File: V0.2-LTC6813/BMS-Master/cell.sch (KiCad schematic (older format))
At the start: 3 parts

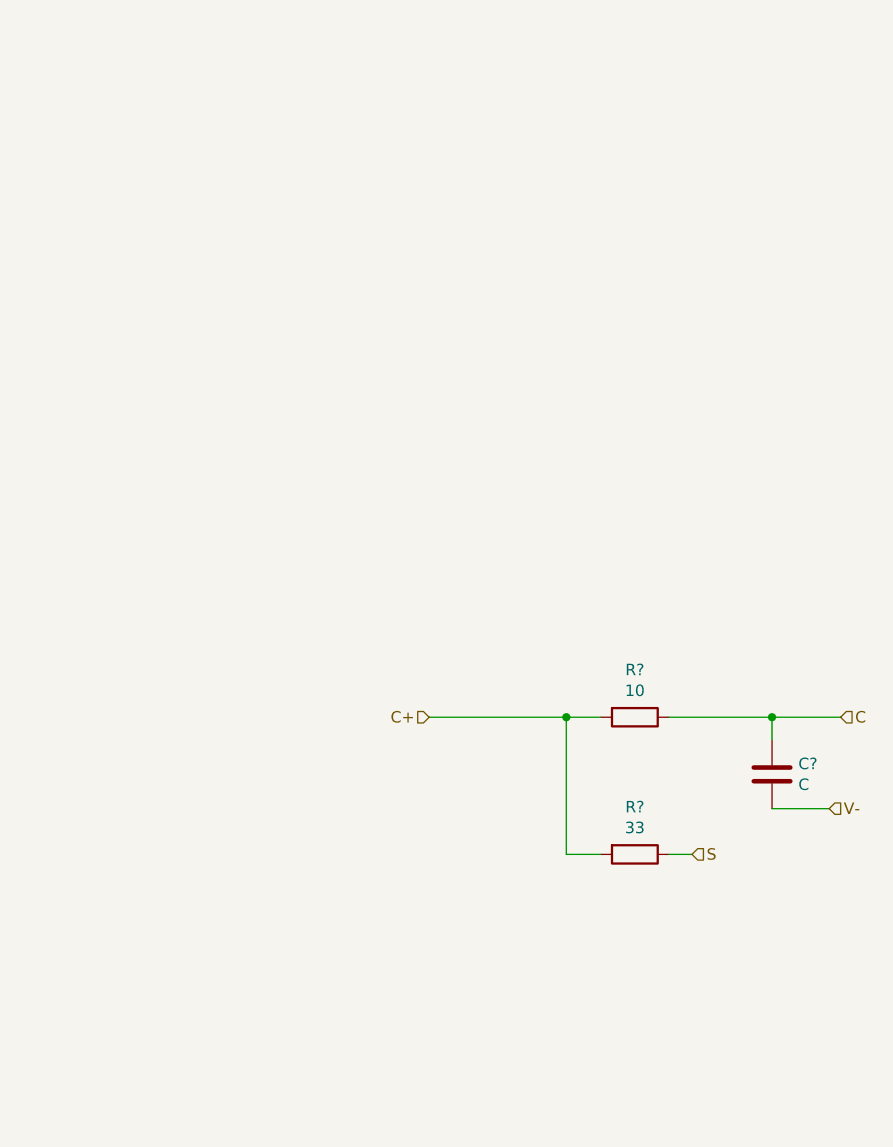
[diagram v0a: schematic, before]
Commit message: schematics 50% complete3d
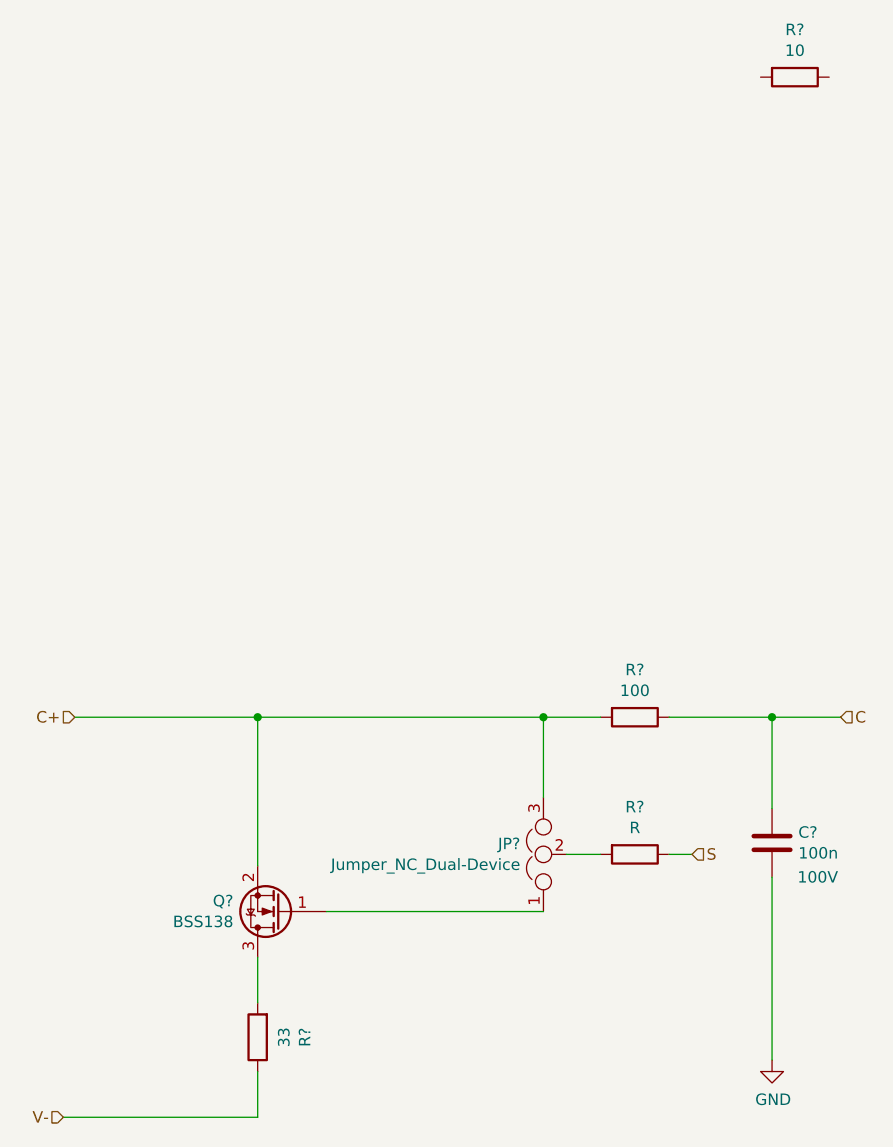
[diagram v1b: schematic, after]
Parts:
- added JP?: Jumper_NC_Dual-Device, symbol BMS-Master-rescue:Jumper_NC_Dual-Device
- added Q?: BSS138, Package_TO_SOT_SMD:SOT-23, symbol Transistor_FET:BSS138
- added R?: 10, Resistor_SMD:R_0603_1608Metric_Pad0.99x1.00mm_HandSolder, symbol Device:R
- added R?: 33, Resistor_SMD:R_0603_1608Metric_Pad0.99x1.00mm_HandSolder, symbol Device:R
- C?: value C -> 100n; Voltage (none) -> 100V
- R?: value 10 -> 100
- R?: value 33 -> R
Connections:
- net C+: now also JP?.3, Q?.2 (S); no longer R?.2
- net V-: now also R?.1; no longer C?.1
- new net: JP?.2, R?.2
- new net: JP?.1, Q?.1 (G)
- new net: Q?.3 (D), R?.2
- new net GND: C?.1
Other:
- moved on the sheet: C?
